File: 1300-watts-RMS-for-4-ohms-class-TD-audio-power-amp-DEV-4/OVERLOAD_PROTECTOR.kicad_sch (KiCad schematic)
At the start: 47 parts, among them Q901 2N5401, Q902 2N5551, Q903 TIP41C, U901 RC4558

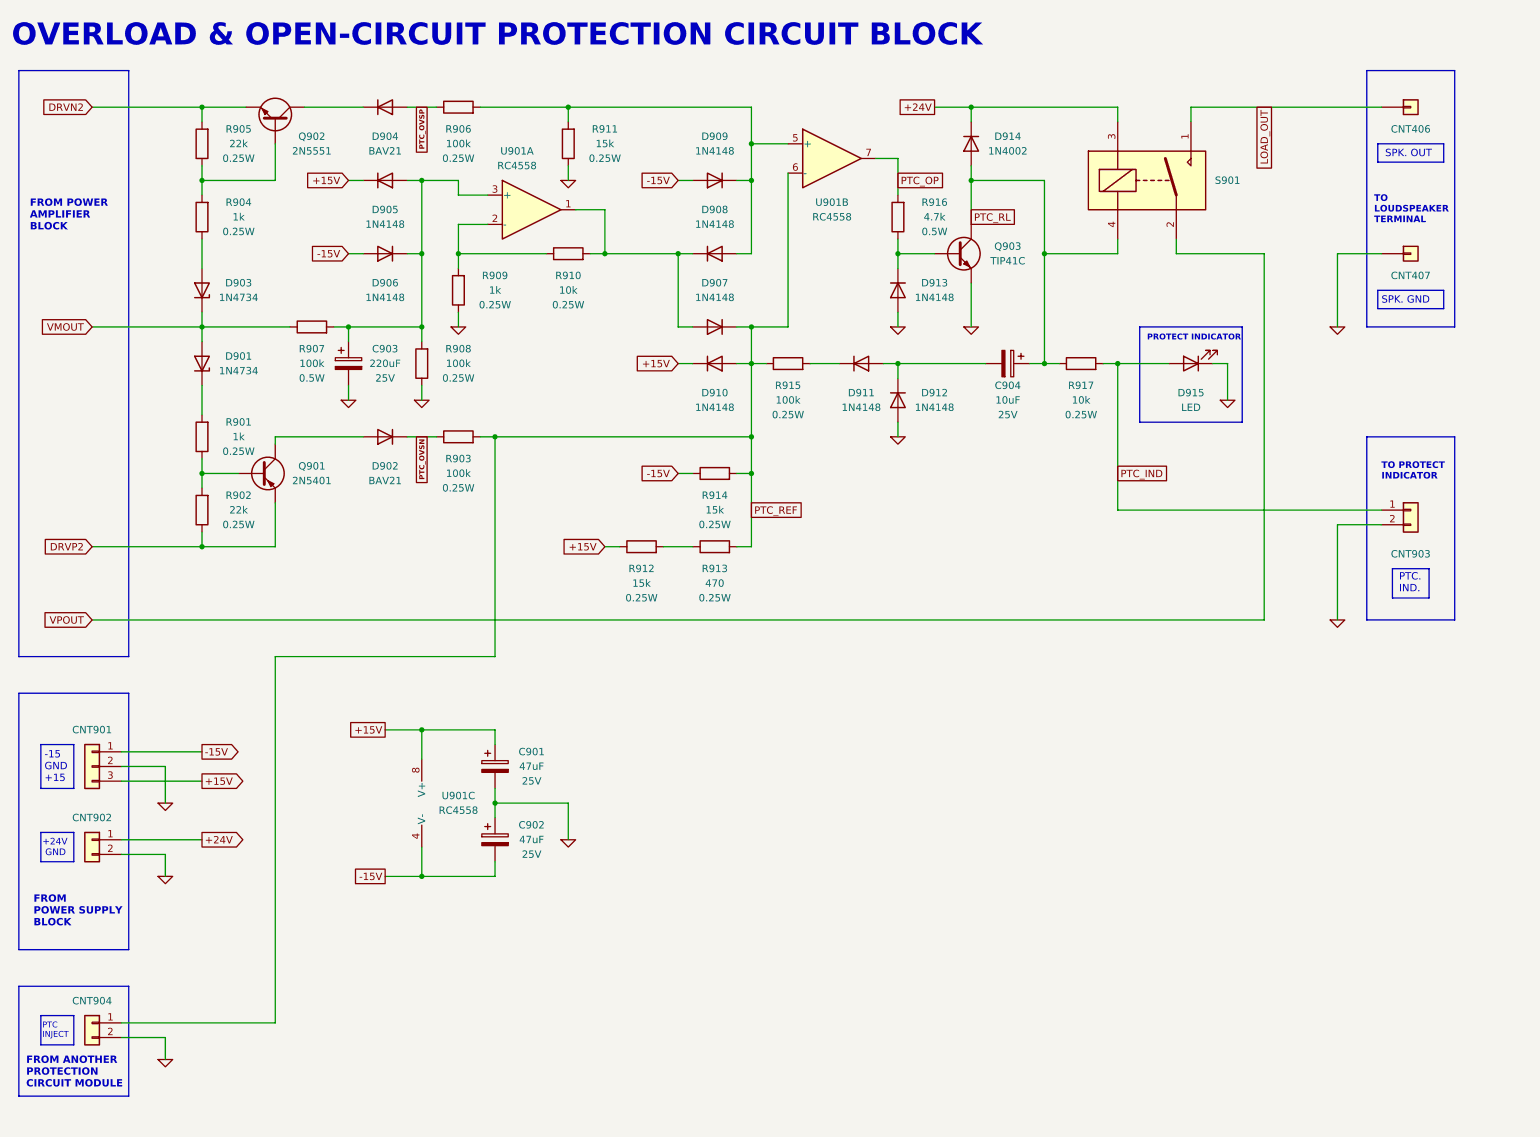
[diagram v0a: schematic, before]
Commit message: Update Wed Sep 14 11:14:32 AM WIB 2022
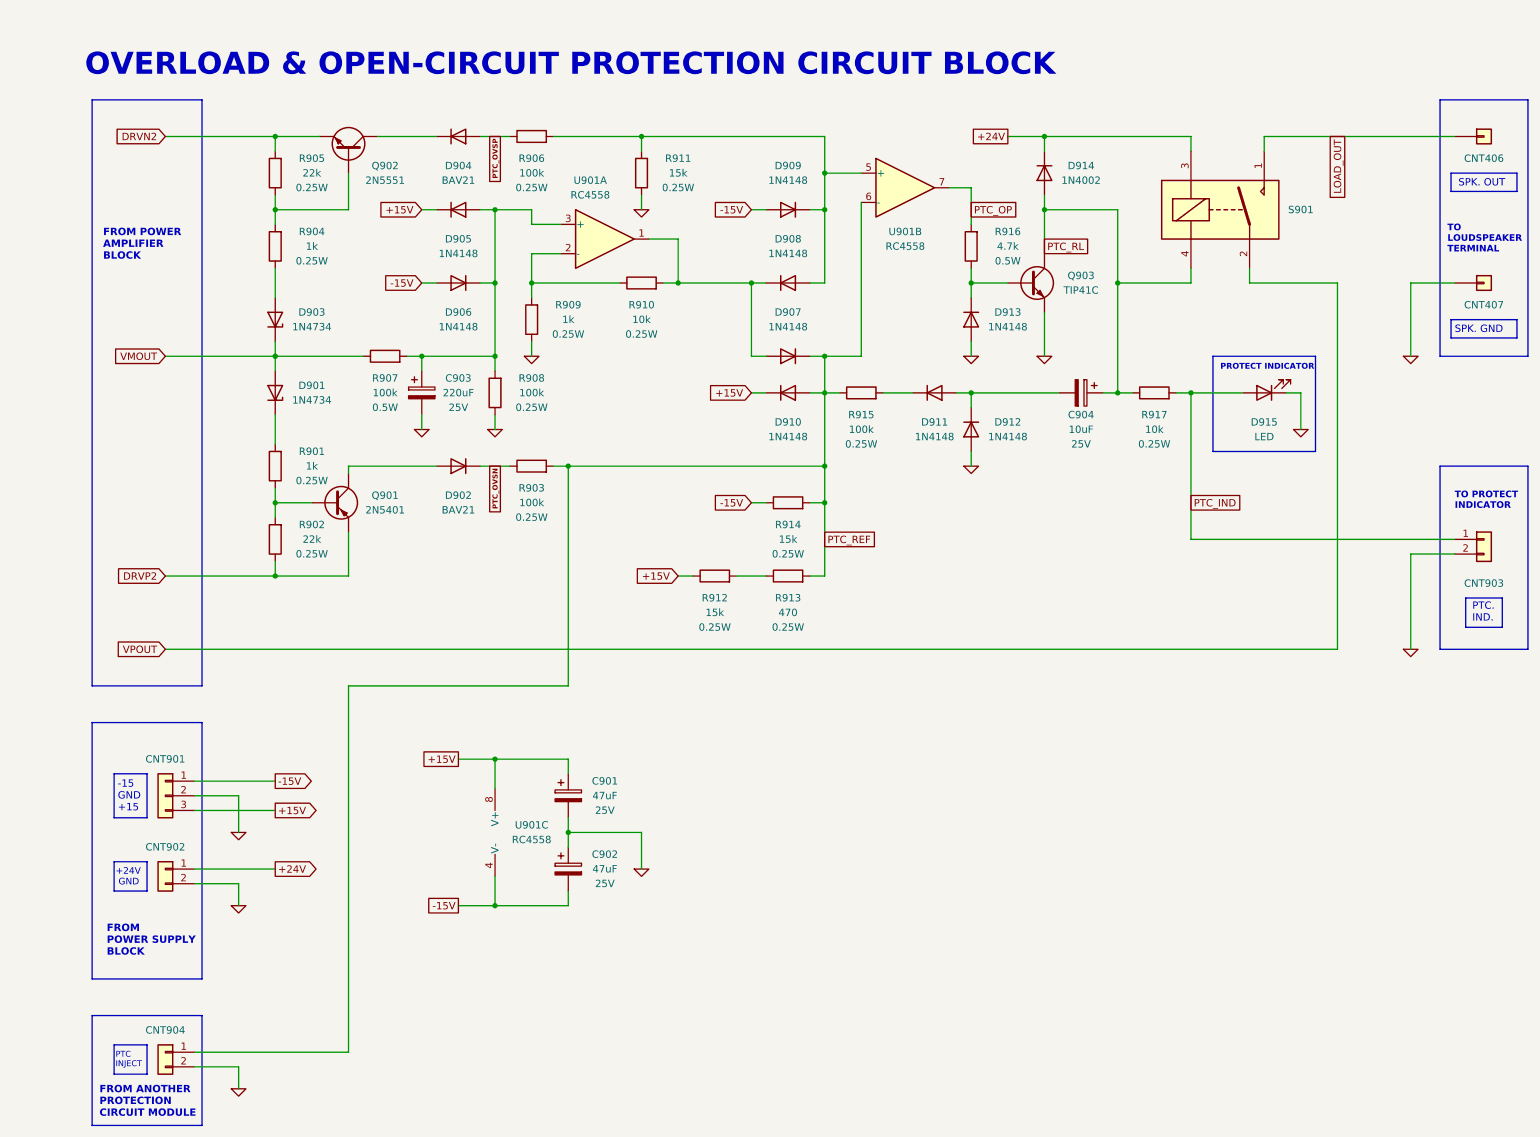
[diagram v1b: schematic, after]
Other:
- moved on the sheet: C901, C902, C903, C904, CNT406, CNT407, CNT901, CNT902, CNT903, CNT904, D901, D902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

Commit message: Update Sat Sep 17 07:48:27 PM WIB 2022
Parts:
- D901, D903: footprint BSD_POWER_AMP:DIODE_ZENER_AXIAL_SMALL_SI -> BSD_POWER_AMP:D_DO-41_SOD81_P10.16mm_Zener_Horizontal
- D902, D904, D905, D906, D907, D908, D909, D910, D911, D912, D913: footprint BSD_POWER_AMP:DIODE_AXIAL_SMALL_GE -> BSD_POWER_AMP:D_DO-35_SOD27_P10.16mm_Horizontal
- D914: footprint BSD_POWER_AMP:DIODE_AXIAL_SMALL_SI -> BSD_POWER_AMP:D_DO-41_SOD81_P10.16mm_Horizontal
- Q901, Q902: footprint BSD_POWER_AMP:TO-92-EBC -> BSD_POWER_AMP:TO-92_Inline_Wide_EBC
- R901, R902, R903, R904, R905, R906, R908, R909, R910, R911, R912, R913, R914, R915, R917: footprint BSD_POWER_AMP:RESISTOR_AXIAL_0.25W -> BSD_POWER_AMP:R_Axial_DIN0207_L6.3mm_D2.5mm_P10.16mm_Horizontal
- R907, R916: footprint BSD_POWER_AMP:RESISTOR_AXIAL_0.5W -> BSD_POWER_AMP:R_Axial_DIN0309_L9.0mm_D3.2mm_P12.70mm_Horizontal
